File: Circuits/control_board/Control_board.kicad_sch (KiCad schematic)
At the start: 66 parts, among them J1 Pic UART JST Connector, Q1 S8050, Q2 S8050, Q3 S8550, Q4 S8050, U1 PC817, U10 PIC18F2550-ISP, U11 LM317_TO-220, U12 MCP41010, U13 7400, U2 PC817, U3 PC817, U4 PC817, U5 TL062, U6 LM393, U7 TL431LP, U8 TL062, U9 LM317_TO-220

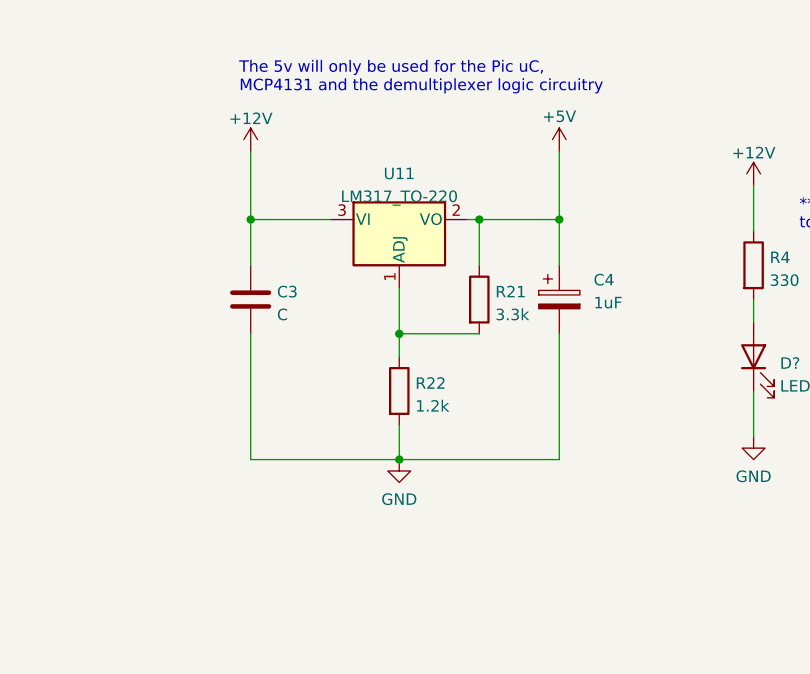
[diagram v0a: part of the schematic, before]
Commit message: minor changes to circuit
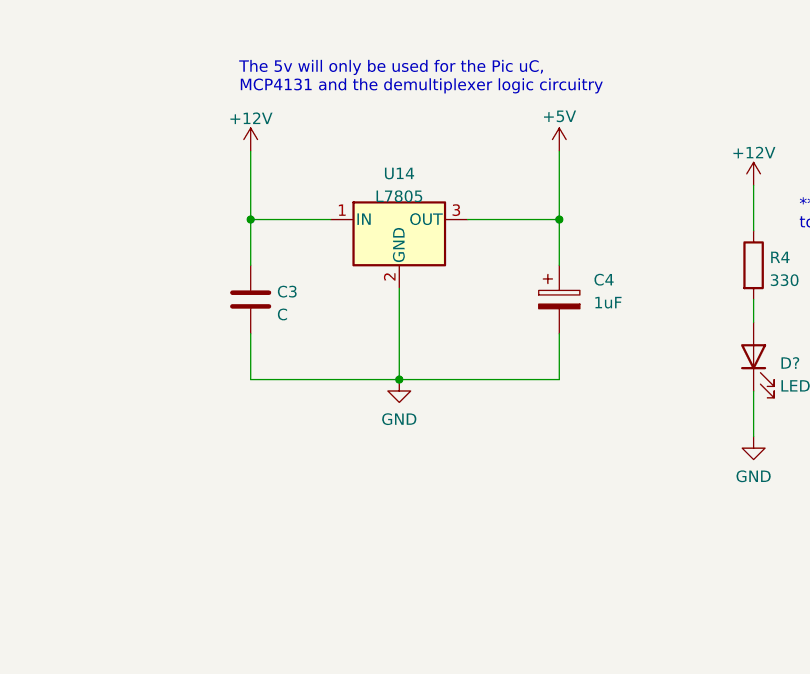
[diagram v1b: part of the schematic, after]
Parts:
- removed R21: 3.3k, Resistor_THT:R_Axial_DIN0207_L6.3mm_D2.5mm_P7.62mm_Horizontal, symbol Device:R
- removed R22: 1.2k, Resistor_THT:R_Axial_DIN0207_L6.3mm_D2.5mm_P7.62mm_Horizontal, symbol Device:R
- removed U11: LM317_TO-220, Package_TO_SOT_THT:TO-220-3_Vertical, symbol Regulator_Linear:LM317_TO-220
- added U14: L7805, symbol Regulator_Linear:L7805
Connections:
- net +12V: now also U14.1 (IN)
- net +5V: now also U14.3 (OUT)
- net GND: now also U14.2 (GND)
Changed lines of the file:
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@@
   (junction (at 406.4 138.43) (diameter 0) (color 0 0 0 0)
   )
-  (junction (at 81.28 -39.37) (diameter 0) (color 0 0 0 0)
-  )
   (junction (at 139.7 -62.23) (diameter 0) (color 0 0 0 0)
   )
@@
   (junction (at 132.08 46.99) (diameter 0) (color 0 0 0 0)
   )
-  (junction (at 72.39 -12.7) (diameter 0) (color 0 0 0 0)
+  (junction (at 72.39 -21.59) (diameter 0) (color 0 0 0 0)
   )
   (junction (at 68.58 127) (diameter 0) (color 0 0 0 0)
@@
   (junction (at 270.51 123.19) (diameter 0) (color 0 0 0 0)
   )
-  (junction (at 72.39 -26.67) (diameter 0) (color 0 0 0 0)
-  )
   (junction (at -127 107.95) (diameter 0) (color 0 0 0 0)
   )
@@
     (stroke (width 0) (type default))
   )
+  (wire (pts (xy 55.88 -26.67) (xy 55.88 -21.59))
+    (stroke (width 0) (type default))
+  )
   (wire (pts (xy 226.06 43.18) (xy 248.92 43.18))
     (stroke (width 0) (type default))
@@
     (stroke (width 0) (type default))
   )
-  (wire (pts (xy 90.17 -12.7) (xy 90.17 -26.67))
-    (stroke (width 0) (type default))
-  )
   (wire (pts (xy 119.38 148.59) (xy 119.38 154.94))
     (stroke (width 0) (type default))
@@
     (stroke (width 0) (type default))
   )
-  (wire (pts (xy 55.88 -26.67) (xy 55.88 -12.7))
+  (wire (pts (xy 72.39 -31.75) (xy 72.39 -21.59))
     (stroke (width 0) (type default))
   )
@@
     (stroke (width 0) (type default))
   )
-  (wire (pts (xy 81.28 -39.37) (xy 80.01 -39.37))
+  (wire (pts (xy 80.01 -39.37) (xy 90.17 -39.37))
     (stroke (width 0) (type default))
   )
@@
     (stroke (width 0) (type default))
   )
-  (wire (pts (xy 72.39 -31.75) (xy 72.39 -26.67))
-    (stroke (width 0) (type default))
-  )
   (wire (pts (xy 157.48 54.61) (xy 160.02 54.61))
     (stroke (width 0) (type default))
@@
     (stroke (width 0) (type default))
   )
-  (wire (pts (xy 81.28 -39.37) (xy 81.28 -34.29))
-    (stroke (width 0) (type default))
-  )
   (wire (pts (xy 124.46 57.15) (xy 124.46 72.39))
     (stroke (width 0) (type default))
@@
     (stroke (width 0) (type default))
   )
-  (wire (pts (xy 90.17 -39.37) (xy 81.28 -39.37))
-    (stroke (width 0) (type default))
-  )
   (wire (pts (xy 66.04 134.62) (xy 66.04 140.97))
     (stroke (width 0) (type default))
@@
     (stroke (width 0) (type default))
   )
-  (wire (pts (xy 55.88 -12.7) (xy 72.39 -12.7))
-    (stroke (width 0) (type default))
-  )
-  (wire (pts (xy 72.39 -26.67) (xy 72.39 -24.13))
+  (wire (pts (xy 55.88 -21.59) (xy 72.39 -21.59))
     (stroke (width 0) (type default))
   )
@@
     (stroke (width 0) (type default))
   )
-  (wire (pts (xy 72.39 -26.67) (xy 81.28 -26.67))
-    (stroke (width 0) (type default))
-  )
   (wire (pts (xy 191.77 -71.12) (xy 191.77 -66.04))
     (stroke (width 0) (type default))
@@
     (stroke (width 0) (type default))
   )
-  (wire (pts (xy 72.39 -16.51) (xy 72.39 -12.7))
-    (stroke (width 0) (type default))
-  )
   (wire (pts (xy 248.92 43.18) (xy 248.92 50.8))
     (stroke (width 0) (type default))
@@
     (stroke (width 0) (type default))
   )
+  (wire (pts (xy 90.17 -26.67) (xy 90.17 -21.59))
+    (stroke (width 0) (type default))
+  )
   (wire (pts (xy 388.62 115.57) (xy 427.99 115.57))
     (stroke (width 0) (type default))
@@
     (stroke (width 0) (type default))
   )
-  (wire (pts (xy 72.39 -12.7) (xy 90.17 -12.7))
+  (wire (pts (xy 72.39 -21.59) (xy 90.17 -21.59))
     (stroke (width 0) (type default))
   )
@@
     )
   )
-  (symbol (lib_id "power:GND") (at 72.39 -12.7 0) (unit 1)
+  (symbol (lib_id "power:GND") (at 72.39 -21.59 0) (unit 1)
     (in_bom yes) (on_board yes) (dnp no) (fields_autoplaced)
-    (property "Reference" "#PWR024" (at 72.39 -6.35 0)
+    (property "Reference" "#PWR024" (at 72.39 -15.24 0)
       (effects (font (size 1.27 1.27)) hide)
     )
-    (property "Value" "GND" (at 72.39 -8.2566 0)
+    (property "Value" "GND" (at 72.39 -17.1466 0)
       (effects (font (size 1.27 1.27)))
     )
-    (property "Footprint" "" (at 72.39 -12.7 0)
+    (property "Footprint" "" (at 72.39 -21.59 0)
       (effects (font (size 1.27 1.27)) hide)
     )
-    (property "Datasheet" "" (at 72.39 -12.7 0)
+    (property "Datasheet" "" (at 72.39 -21.59 0)
       (effects (font (size 1.27 1.27)) hide)
     )
@@
     )
   )
-  (symbol (lib_id "Regulator_Linear:LM317_TO-220") (at 72.39 -39.37 0) (unit 1)
-    (in_bom yes) (on_board yes) (dnp no) (fields_autoplaced)
-    (property "Reference" "U11" (at 72.39 -44.45 0)
-      (effects (font (size 1.27 1.27)))
-    )
-    (property "Value" "LM317_TO-220" (at 72.39 -41.91 0)
-      (effects (font (size 1.27 1.27)))
-    )
-    (property "Footprint" "Package_TO_SOT_THT:TO-220-3_Vertical" (at 72.39 -45.72 0)
-      (effects (font (size 1.27 1.27) italic) hide)
-    )
-    (property "Datasheet" "http://www.ti.com/lit/ds/symlink/lm317.pdf" (at 72.39 -39.37 0)
-      (effects (font (size 1.27 1.27)) hide)
-    )
-    (pin "1")
-    (pin "2")
-    (pin "3")
-    (instances
-      (project "Control_board"
-        (path "/e63e39d7-6ac0-4ffd-8aa3-1841a4541b55"
-          (reference "U11") (unit 1)
-        )
-      )
-    )
-  )
   (symbol (lib_id "Device:R") (at 111.76 -34.29 0) (unit 1)
     (in_bom yes) (on_board yes) (dnp no) (fields_autoplaced)
@@
     )
   )
-  (symbol (lib_id "Device:R") (at 72.39 -20.32 0) (unit 1)
-    (in_bom yes) (on_board yes) (dnp no) (fields_autoplaced)
-    (property "Reference" "R22" (at 74.168 -21.1547 0)
-      (effects (font (size 1.27 1.27)) (justify left))
-    )
-    (property "Value" "1.2k" (at 74.168 -18.6178 0)
-      (effects (font (size 1.27 1.27)) (justify left))
-    )
-    (property "Footprint" "Resistor_THT:R_Axial_DIN0207_L6.3mm_D2.5mm_P7.62mm_Horizontal" (at 70.612 -20.32 90)
-      (effects (font (size 1.27 1.27)) hide)
-    )
-    (property "Datasheet" "~" (at 72.39 -20.32 0)
-      (effects (font (size 1.27 1.27)) hide)
-    )
-    (pin "1")
-    (pin "2")
-    (instances
-      (project "Control_board"
-        (path "/e63e39d7-6ac0-4ffd-8aa3-1841a4541b55"
-          (reference "R22") (unit 1)
-        )
-      )
-    )
-  )
   (symbol (lib_id "power:+5V") (at -127 95.25 0) (unit 1)
     (in_bom yes) (on_board yes) (dnp no) (fields_autoplaced)
@@
     )
   )
-  (symbol (lib_id "Device:R") (at 81.28 -30.48 0) (unit 1)
-    (in_bom yes) (on_board yes) (dnp no) (fields_autoplaced)
-    (property "Reference" "R21" (at 83.058 -31.3147 0)
-      (effects (font (size 1.27 1.27)) (justify left))
-    )
-    (property "Value" "3.3k" (at 83.058 -28.7778 0)
-      (effects (font (size 1.27 1.27)) (justify left))
-    )
-    (property "Footprint" "Resistor_THT:R_Axial_DIN0207_L6.3mm_D2.5mm_P7.62mm_Horizontal" (at 79.502 -30.48 90)
-      (effects (font (size 1.27 1.27)) hide)
-    )
-    (property "Datasheet" "~" (at 81.28 -30.48 0)
-      (effects (font (size 1.27 1.27)) hide)
-    )
-    (pin "1")
-    (pin "2")
-    (instances
-      (project "Control_board"
-        (path "/e63e39d7-6ac0-4ffd-8aa3-1841a4541b55"
-          (reference "R21") (unit 1)
-        )
-      )
-    )
-  )
   (symbol (lib_id "Device:R") (at -55.88 109.22 180) (unit 1)
     (in_bom yes) (on_board yes) (dnp no) (fields_autoplaced)
@@
         )
       )
+    )
+  )
+  (symbol (lib_id "Regulator_Linear:L7805") (at 72.39 -39.37 0) (unit 1)
+    (in_bom yes) (on_board yes) (dnp no) (fields_autoplaced)
+    (property "Reference" "U14" (at 72.39 -44.45 0)
+      (effects (font (size 1.27 1.27)))
+    )
+    (property "Value" "L7805" (at 72.39 -41.91 0)
+      (effects (font (size 1.27 1.27)))
+    )
+    (property "Footprint" "" (at 73.025 -35.56 0)
+      (effects (font (size 1.27 1.27) italic) (justify left) hide)
+    )
+    (property "Datasheet" "http://www.st.com/content/ccc/resource/technical/document/datasheet/41/4f/b3/b0/12/d4/47/88/CD00000444.pdf/files/CD00000444.pdf/jcr:content/translations/en.CD00000444.pdf" (at 72.39 -38.1 0)
+      (effects (font (size 1.27 1.27)) hide)
+    )
+    (pin "1")
+    (pin "2")
+    (pin "3")
+    (instances
+      (project "Control_board"
+        (path "/e63e39d7-6ac0-4ffd-8aa3-1841a4541b55"
+          (reference "U14") (unit 1)
+        )
+      )
